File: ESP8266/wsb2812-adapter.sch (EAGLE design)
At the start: 6 parts, among them CON1 USBMICRO-NO_CENTER

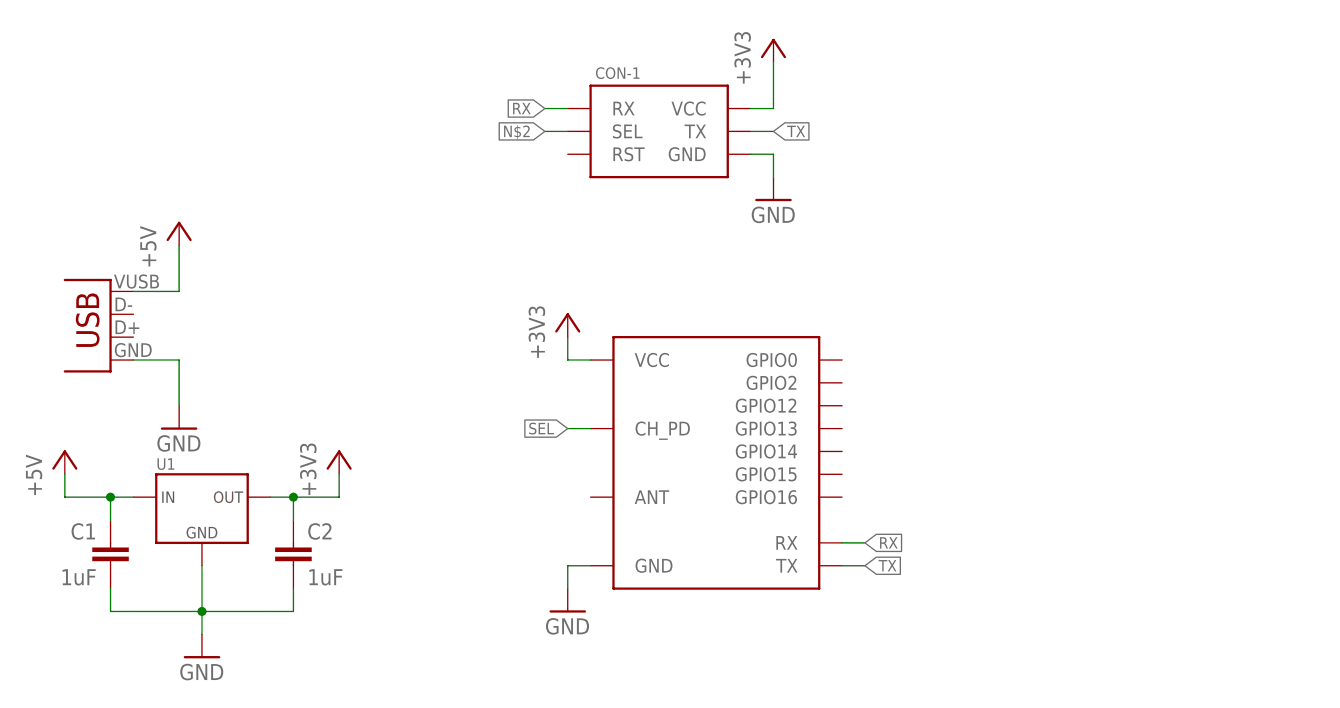
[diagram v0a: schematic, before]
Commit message: V0.1 done
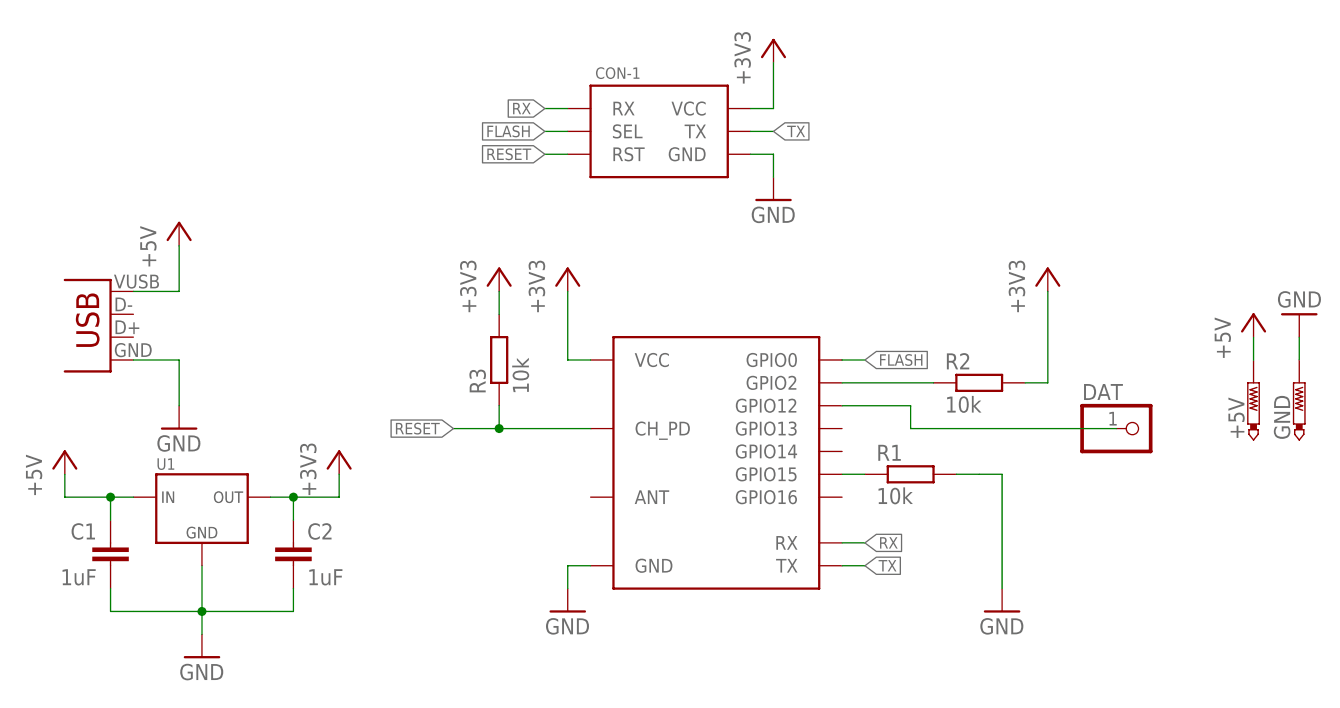
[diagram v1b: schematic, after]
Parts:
- added +5V, GND: PTR1PAD1-20, testpad:PTR1PAD1-20
- added DAT: (no value), pinhead:PINHD-1X1
- added R1, R2, R3: 10k, p.peter-rcl:R-EU_R0603
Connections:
- removed net SEL: U$1.CH_PD
- new net FLASH: CON-1.SEL, U$1.GPIO0
- new net N$1: R1.1, U$1.GPIO15
- new net N$3: R2.1, U$1.GPIO2
- new net RESET: CON-1.RST, R3.1, U$1.CH_PD
- net +3V3: now also R2.2, R3.2
- net +5V: now also +5V.TP
- net GND: now also GND.TP, R1.2
- net N$2: now also DAT.1, U$1.GPIO12; no longer CON-1.SEL
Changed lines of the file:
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@@
 <?xml version="1.0" encoding="utf-8"?>
 <!DOCTYPE eagle SYSTEM "eagle.dtd">
-<eagle version="7.1.0">
+<eagle version="7.3.0">
 <drawing>
 <settings>
@@
 <part name="+3V3" library="supply1" deviceset="+3V3" device=""/>
 <part name="GND4" library="supply1" deviceset="GND" device=""/>
+<part name="R1" library="p.peter-rcl" deviceset="R-EU_" device="R0603" value="10k"/>
+<part name="GND5" library="supply1" deviceset="GND" device=""/>
+<part name="R2" library="p.peter-rcl" deviceset="R-EU_" device="R0603" value="10k"/>
+<part name="+3V4" library="supply1" deviceset="+3V3" device=""/>
+<part name="R3" library="p.peter-rcl" deviceset="R-EU_" device="R0603" value="10k"/>
+<part name="+3V5" library="supply1" deviceset="+3V3" device=""/>
+<part name="+5V" library="testpad" deviceset="PTR1" device="PAD1-20"/>
+<part name="GND" library="testpad" deviceset="PTR1" device="PAD1-20"/>
+<part name="DAT" library="pinhead" deviceset="PINHD-1X1" device=""/>
+<part name="P+3" library="supply1" deviceset="+5V" device=""/>
+<part name="GND6" library="supply1" deviceset="GND" device=""/>
 </parts>
 <sheets>
@@
 <instance part="P+2" gate="1" x="-17.78" y="68.58"/>
 <instance part="GND3" gate="1" x="25.4" y="25.4"/>
-<instance part="+3V2" gate="G$1" x="25.4" y="58.42"/>
+<instance part="+3V2" gate="G$1" x="25.4" y="63.5"/>
 <instance part="+3V3" gate="G$1" x="48.26" y="88.9"/>
 <instance part="GND4" gate="1" x="48.26" y="71.12"/>
+<instance part="R1" gate="G$1" x="63.5" y="40.64"/>
+<instance part="GND5" gate="1" x="73.66" y="25.4"/>
+<instance part="R2" gate="G$1" x="71.12" y="50.8"/>
+<instance part="+3V4" gate="G$1" x="78.74" y="63.5"/>
+<instance part="R3" gate="G$1" x="17.78" y="53.34" rot="R90"/>
+<instance part="+3V5" gate="G$1" x="17.78" y="63.5"/>
+<instance part="+5V" gate="G$1" x="101.6" y="50.8"/>
+<instance part="GND" gate="G$1" x="106.68" y="50.8"/>
+<instance part="DAT" gate="G$1" x="88.9" y="45.72"/>
+<instance part="P+3" gate="1" x="101.6" y="58.42"/>
+<instance part="GND6" gate="1" x="106.68" y="58.42" rot="R180"/>
 </instances>
 <busses>
@@
 <pinref part="P+2" gate="1" pin="+5V"/>
 </segment>
+<segment>
+<pinref part="+5V" gate="G$1" pin="TP"/>
+<pinref part="P+3" gate="1" pin="+5V"/>
+<wire x1="101.6" y1="55.88" x2="101.6" y2="53.34" width="0.1524" layer="91"/>
+</segment>
 </net>
 <net name="+3V3" class="0">
@@
 <pinref part="U$1" gate="G$1" pin="VCC"/>
 <wire x1="27.94" y1="53.34" x2="25.4" y2="53.34" width="0.1524" layer="91"/>
-<wire x1="25.4" y1="53.34" x2="25.4" y2="55.88" width="0.1524" layer="91"/>
+<wire x1="25.4" y1="53.34" x2="25.4" y2="60.96" width="0.1524" layer="91"/>
 <pinref part="+3V2" gate="G$1" pin="+3V3"/>
 </segment>
@@
 <wire x1="48.26" y1="81.28" x2="48.26" y2="86.36" width="0.1524" layer="91"/>
 <pinref part="+3V3" gate="G$1" pin="+3V3"/>
+</segment>
+<segment>
+<pinref part="R2" gate="G$1" pin="2"/>
+<wire x1="76.2" y1="50.8" x2="78.74" y2="50.8" width="0.1524" layer="91"/>
+<wire x1="78.74" y1="50.8" x2="78.74" y2="60.96" width="0.1524" layer="91"/>
+<pinref part="+3V4" gate="G$1" pin="+3V3"/>
+</segment>
+<segment>
+<pinref part="R3" gate="G$1" pin="2"/>
+<pinref part="+3V5" gate="G$1" pin="+3V3"/>
+<wire x1="17.78" y1="60.96" x2="17.78" y2="58.42" width="0.1524" layer="91"/>
 </segment>
 </net>
@@
 <pinref part="GND4" gate="1" pin="GND"/>
 </segment>
-</net>
-<net name="SEL" class="0">
-<segment>
-<pinref part="U$1" gate="G$1" pin="CH_PD"/>
-<wire x1="27.94" y1="45.72" x2="25.4" y2="45.72" width="0.1524" layer="91"/>
-<label x="25.4" y="45.72" size="1.27" layer="95" rot="R180" xref="yes"/>
+<segment>
+<pinref part="R1" gate="G$1" pin="2"/>
+<wire x1="68.58" y1="40.64" x2="71.12" y2="40.64" width="0.1524" layer="91"/>
+<wire x1="71.12" y1="40.64" x2="73.66" y2="40.64" width="0.1524" layer="91"/>
+<wire x1="73.66" y1="40.64" x2="73.66" y2="27.94" width="0.1524" layer="91"/>
+<pinref part="GND5" gate="1" pin="GND"/>
+</segment>
+<segment>
+<pinref part="GND" gate="G$1" pin="TP"/>
+<pinref part="GND6" gate="1" pin="GND"/>
+<wire x1="106.68" y1="55.88" x2="106.68" y2="53.34" width="0.1524" layer="91"/>
 </segment>
 </net>
@@
 </segment>
 </net>
-<net name="N$2" class="0">
+<net name="FLASH" class="0">
+<segment>
+<pinref part="U$1" gate="G$1" pin="GPIO0"/>
+<wire x1="55.88" y1="53.34" x2="58.42" y2="53.34" width="0.1524" layer="91"/>
+<label x="58.42" y="53.34" size="1.27" layer="95" ratio="12" xref="yes"/>
+</segment>
 <segment>
 <pinref part="CON-1" gate="G$1" pin="SEL"/>
@@
 </segment>
 </net>
+<net name="RESET" class="0">
+<segment>
+<pinref part="CON-1" gate="G$1" pin="RST"/>
+<wire x1="25.4" y1="76.2" x2="22.86" y2="76.2" width="0.1524" layer="91"/>
+<label x="22.86" y="76.2" size="1.27" layer="95" ratio="12" rot="R180" xref="yes"/>
+</segment>
+<segment>
+<pinref part="U$1" gate="G$1" pin="CH_PD"/>
+<wire x1="27.94" y1="45.72" x2="17.78" y2="45.72" width="0.1524" layer="91"/>
+<label x="12.7" y="45.72" size="1.27" layer="95" rot="R180" xref="yes"/>
+<pinref part="R3" gate="G$1" pin="1"/>
+<wire x1="17.78" y1="45.72" x2="12.7" y2="45.72" width="0.1524" layer="91"/>
+<wire x1="17.78" y1="48.26" x2="17.78" y2="45.72" width="0.1524" layer="91"/>
+<junction x="17.78" y="45.72"/>
+</segment>
+</net>
+<net name="N$1" class="0">
+<segment>
+<pinref part="U$1" gate="G$1" pin="GPIO15"/>
+<pinref part="R1" gate="G$1" pin="1"/>
+<wire x1="55.88" y1="40.64" x2="58.42" y2="40.64" width="0.1524" layer="91"/>
+</segment>
+</net>
+<net name="N$3" class="0">
+<segment>
+<pinref part="U$1" gate="G$1" pin="GPIO2"/>
+<pinref part="R2" gate="G$1" pin="1"/>
+<wire x1="66.04" y1="50.8" x2="55.88" y2="50.8" width="0.1524" layer="91"/>
+</segment>
+</net>
+<net name="N$2" class="0">
+<segment>
+<pinref part="U$1" gate="G$1" pin="GPIO12"/>
+<wire x1="55.88" y1="48.26" x2="63.5" y2="48.26" width="0.1524" layer="91"/>
+<wire x1="63.5" y1="48.26" x2="63.5" y2="45.72" width="0.1524" layer="91"/>
+<pinref part="DAT" gate="G$1" pin="1"/>
+<wire x1="63.5" y1="45.72" x2="86.36" y2="45.72" width="0.1524" layer="91"/>
+</segment>
+</net>
